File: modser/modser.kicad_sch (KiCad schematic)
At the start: 3 parts, among them IC1 AS5600-ASOT, U1 DRV8313PWPR, U2 XIAO-RP2040-DIP

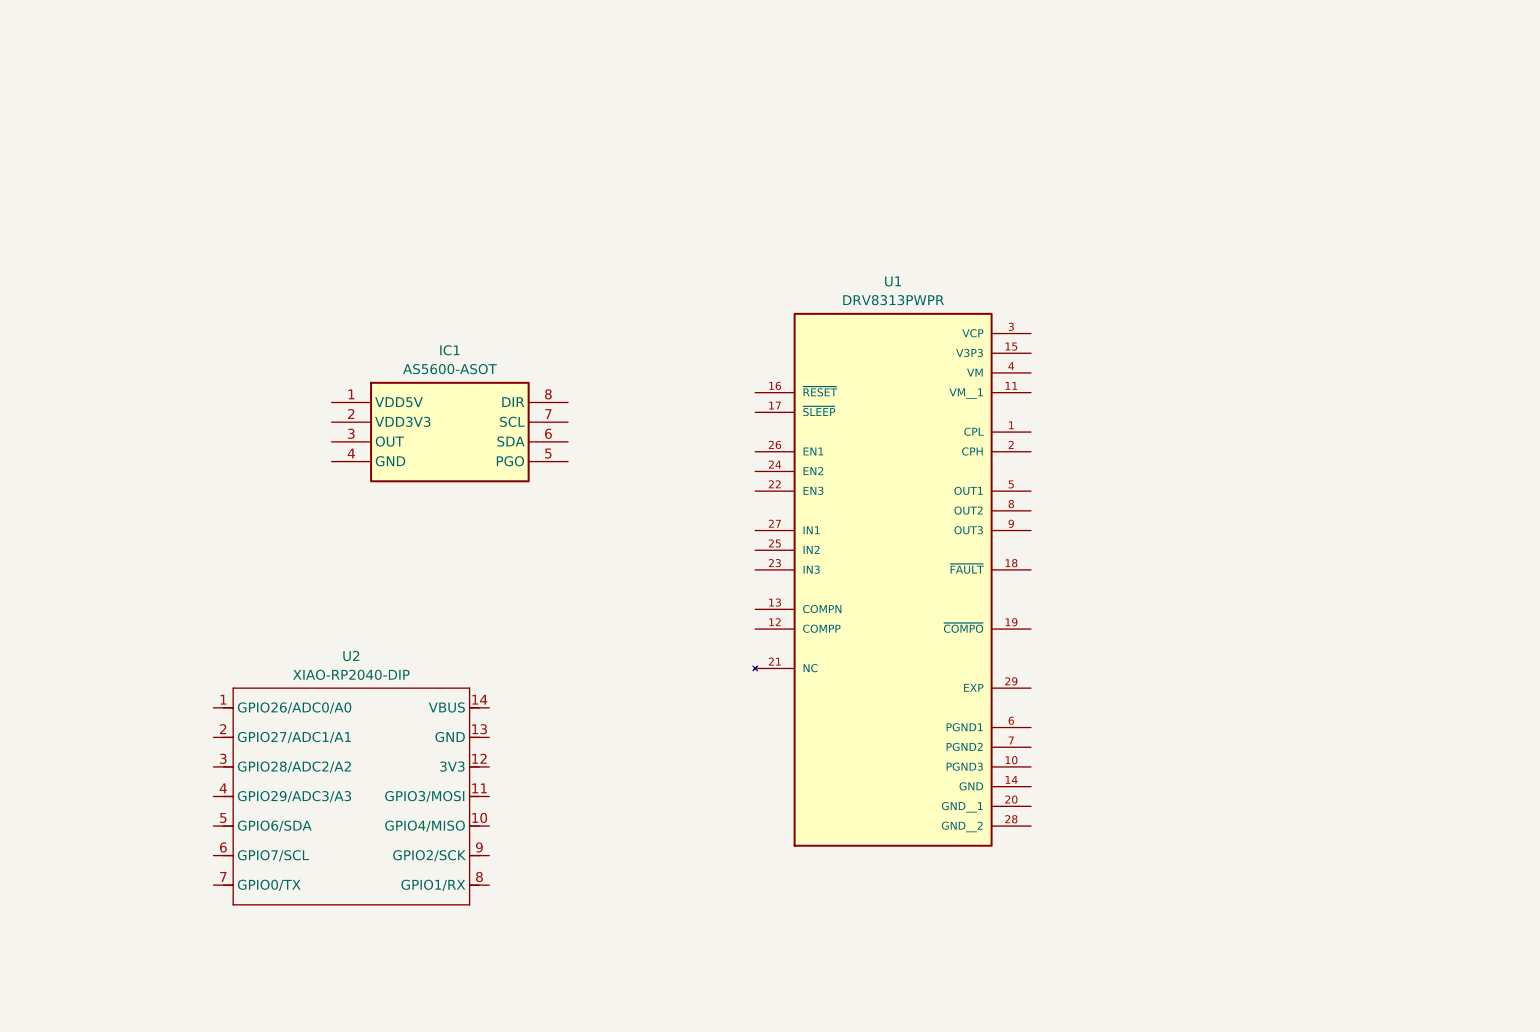
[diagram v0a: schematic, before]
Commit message: Schematic draft complete!
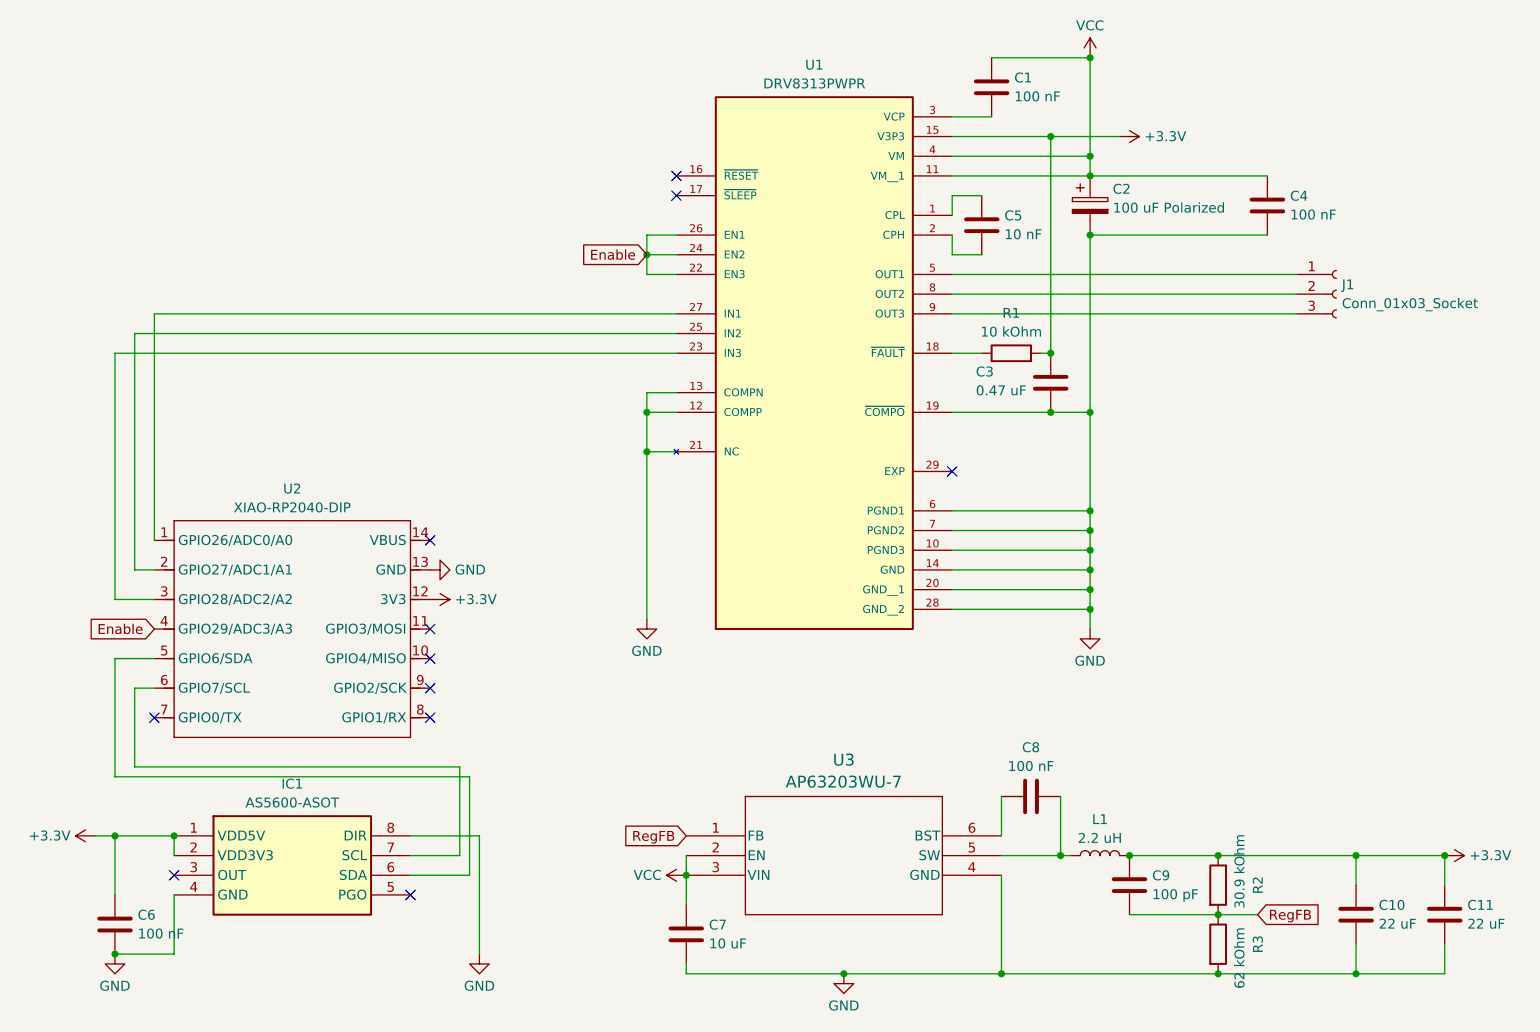
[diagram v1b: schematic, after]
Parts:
- added C1, C4, C6, C8: 100 nF, symbol Device:C
- added C10, C11: 22 uF, symbol Device:C
- added C2: 100 uF Polarized, symbol Device:C_Polarized
- added C3: 0.47 uF, symbol Device:C
- added C5: 10 nF, symbol Device:C
- added C7: 10 uF, symbol Device:C
- added C9: 100 pF, symbol Device:C
- added J1: Conn_01x03_Socket, symbol Connector:Conn_01x03_Socket
- added L1: 2.2 uH, symbol Device:L
- added R1: 10 kOhm, symbol Device:R
- added R2: 30.9 kOhm, symbol Device:R
- added R3: 62 kOhm, symbol Device:R
- added U3: AP63203WU-7, LIB_AP63203WU-7:AP63203WU7, symbol 2025-08-06_01-37-09:AP63203WU-7
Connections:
- net +3.3V: now reaches IC1.1 (VDD5V)
- net +3.3V: now also IC1.2 (VDD3V3), U1.15 (V3P3), U2.12 (3V3), C10.1, C11.1, C3.2, C6.1, C9.1, L1.2, R1.2, R2.1
- net GND: now reaches IC1.4 (GND)
- net GND: now also IC1.8 (DIR), U1.10 (PGND3), U1.12 (COMPP), U1.13 (COMPN), U1.14 (GND), U1.19 (~{COMPO}), U1.20 (GND__1), U1.21 (NC), U1.28 (GND__2), U1.6 (PGND1), U1.7 (PGND2), U2.13 (GND), C10.2, C11.2, C2.2, C3.1, C4.2, C6.2, C7.2, R3.2, U3.4 (GND)
- net at IC1.6 (SDA): now also U2.5 (GPIO6/SDA)
- net at IC1.7 (SCL): now also U2.6 (GPIO7/SCL)
- net at U2.1 (GPIO26/ADC0/A0): now also U1.27 (IN1)
- net at U2.2 (GPIO27/ADC1/A1): now also U1.25 (IN2)
- net at U2.3 (GPIO28/ADC2/A2): now also U1.23 (IN3)
- net Enable: now reaches U2.4 (GPIO29/ADC3/A3)
- net Enable: now also U1.22 (EN3), U1.24 (EN2), U1.26 (EN1)
- net at U1.1 (CPL): now also C5.1
- net VCC: now reaches U1.11 (VM__1)
- net VCC: now also U1.4 (VM), C1.1, C2.1, C4.1, C7.1, U3.2 (EN), U3.3 (VIN)
- net at U1.18 (~{FAULT}): now also R1.1
- net at U1.2 (CPH): now also C5.2
- net at U1.3 (VCP): now also C1.2
- net at U1.5 (OUT1): now also J1.1 (Pin_1)
- net at U1.8 (OUT2): now also J1.2 (Pin_2)
- net at U1.9 (OUT3): now also J1.3 (Pin_3)
- new net: C8.2, L1.1, U3.5 (SW)
- new net: C8.1, U3.6 (BST)
- new net RegFB: C9.2, R2.2, R3.1, U3.1 (FB)
- no-connect marks 0 -> 11
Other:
- moved on the sheet: IC1, U1, U2
